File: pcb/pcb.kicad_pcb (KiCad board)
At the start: 4 copper layers, 69 x 25.5 mm, 30 parts, among them J1 Conn_01x02_Pin, J2 Conn_01x08_Pin, J3 Conn_01x02_Pin, U1 ATtiny85-20P, U2 FS8205A, U3 TP4056, U4 DW01A, U5 AMS1117-5.0

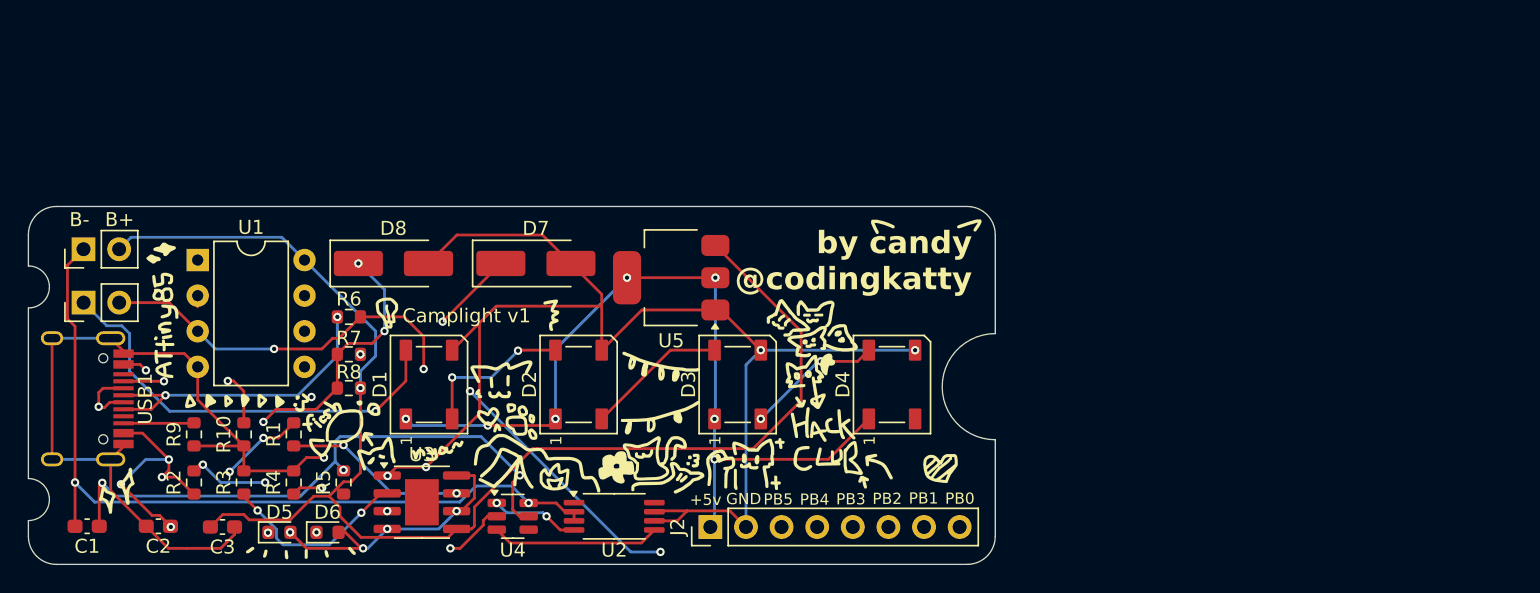
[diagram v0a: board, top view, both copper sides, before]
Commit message: add stuffu
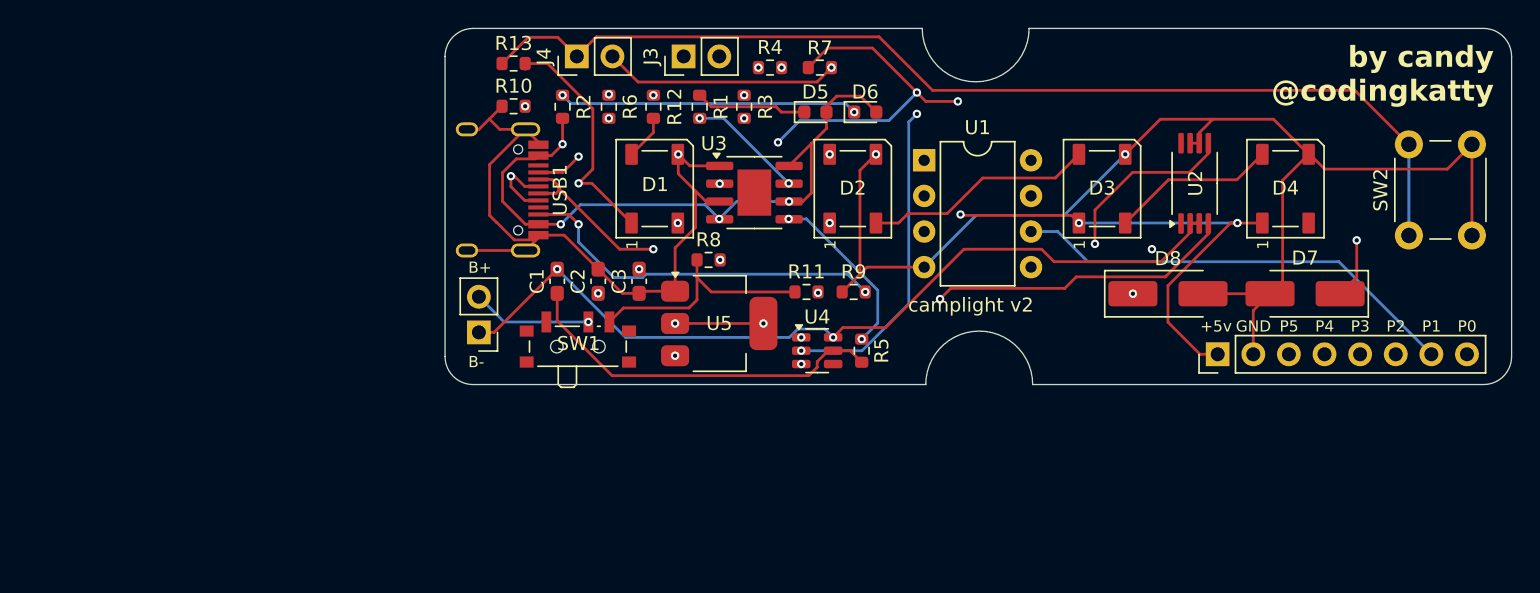
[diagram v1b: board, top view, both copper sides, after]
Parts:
- added J4: Conn_01x02_Pin, Connector_PinHeader_2.54mm:PinHeader_1x02_P2.54mm_Vertical, F.Cu at (94.4, 40.1)
- added R11: 10k, Resistor_SMD:R_0603_1608Metric, F.Cu at (110.7, 56.9)
- added R12: 470, Resistor_SMD:R_0603_1608Metric, F.Cu at (99.8, 43.7)
- added R13: 4.7k, Resistor_SMD:R_0603_1608Metric, F.Cu at (89.9, 40.6)
- added SW1: SW_SPDT, Button_Switch_SMD:SW_SPDT_PCM12, F.Cu at (94.4, 60.5)
- added SW2: SW_Push, Button_Switch_THT:SW_PUSH_6mm, F.Cu at (153.7, 52.9)
- moved D8 55.3 mm to (136.5, 57.0)
- moved D7 54.9 mm to (146.3, 57.0), turned to 180 degrees
- moved U1 52.3 mm to (119.1, 47.5)
- moved D6 48.7 mm to (114.9, 44.1)
- moved D5 48.6 mm to (111.4, 44.1)
- moved R9 48.1 mm to (114.1, 56.9), turned to 0 degrees
- moved U2 47.7 mm to (138.4, 49.1), turned to 90 degrees
- moved J3 46.3 mm to (102.0, 40.1)
- moved R4 45.1 mm to (108.1, 40.9), turned to 0 degrees
- moved R3 44.6 mm to (106.3, 43.7)
- moved R7 39.3 mm to (111.7, 40.9)
- moved J2 38.2 mm to (140.1, 61.3)
- moved R5 38.1 mm to (114.7, 61.1), turned to -90 degrees
- moved C1 37.8 mm to (93.0, 56.1), turned to 90 degrees
- moved R2 37.5 mm to (93.3, 43.7)
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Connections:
- C3 pad 2: OUT+ -> Net-(J1-Pin_2)
- J1 pad 2: OUT+ -> Net-(J1-Pin_2)
- J3 pad 1: Net-(D1-DIN) -> Net-(J3-Pin_1)
- R5 pad 1: OUT+ -> Net-(J1-Pin_2)
- U1 pad 8: OUT+ -> Net-(U1-VCC)
- U3 pad 5: OUT+ -> Net-(J1-Pin_2)
- U5 pad 3: OUT+ -> Net-(U1-VCC)
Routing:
- net OUT+: track 98.3 -> 17.2 mm, vias 1 -> 0
- net Net-(J4-Pin_1): track 0.00 -> 76.3 mm
- net D+: track 36.1 -> 77.0 mm
- net Net-(J1-Pin_2): track 0.00 -> 38.8 mm, vias 0 -> 4
- net D-: track 35.4 -> 72.2 mm, vias 4 -> 6
- net Net-(U1-VCC): track 0.00 -> 36.2 mm, vias 0 -> 2
- net +5V: track 59.7 -> 90.8 mm
- net Net-(D1-DIN): track 30.9 -> 3.21 mm, vias 1 -> 0
- net Net-(U2-G1): track 6.31 -> 32.8 mm
- net Net-(U2-G2): track 12.0 -> 38.2 mm, vias 0 -> 2
- net Net-(USB1-CC2): track 5.04 -> 26.5 mm, vias 0 -> 2
- net Net-(J2-Pin_7): track 51.4 -> 32.2 mm, vias 2 -> 0
- net Net-(U4-CS): track 17.6 -> 36.3 mm, vias 2 -> 3
- net Net-(J2-Pin_3): track 51.7 -> 33.3 mm
- net Net-(J2-Pin_6): track 48.5 -> 30.7 mm
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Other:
- board size 69 x 25.5 mm -> 76.1 x 25.4 mm
- board text added: "P0"
- board text added: "P1"
- board text added: "P2"
- board text added: "P3"
- board text added: "P4"
- board text added: "P5"
- board text added: "camplight v2"
- board text removed: "Camplight v1"
- board text removed: "PB0"
- board text removed: "PB1"
- board text removed: "PB2"
- board text removed: "PB3"
- board text removed: "PB4"
- board text removed: "PB5"
- board text removed: "meow, what brings you here at the back? :3"
